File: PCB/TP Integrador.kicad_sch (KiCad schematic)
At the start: 33 parts, among them Q1 BC547C, Q10 BC547C, Q11 BC547C, Q2 2N3019, Q3 D45H11, Q4 BC547C, Q5 BC557C, Q6 BC557C, Q7 BC547C, Q8 BC557C, Q9 BC547C

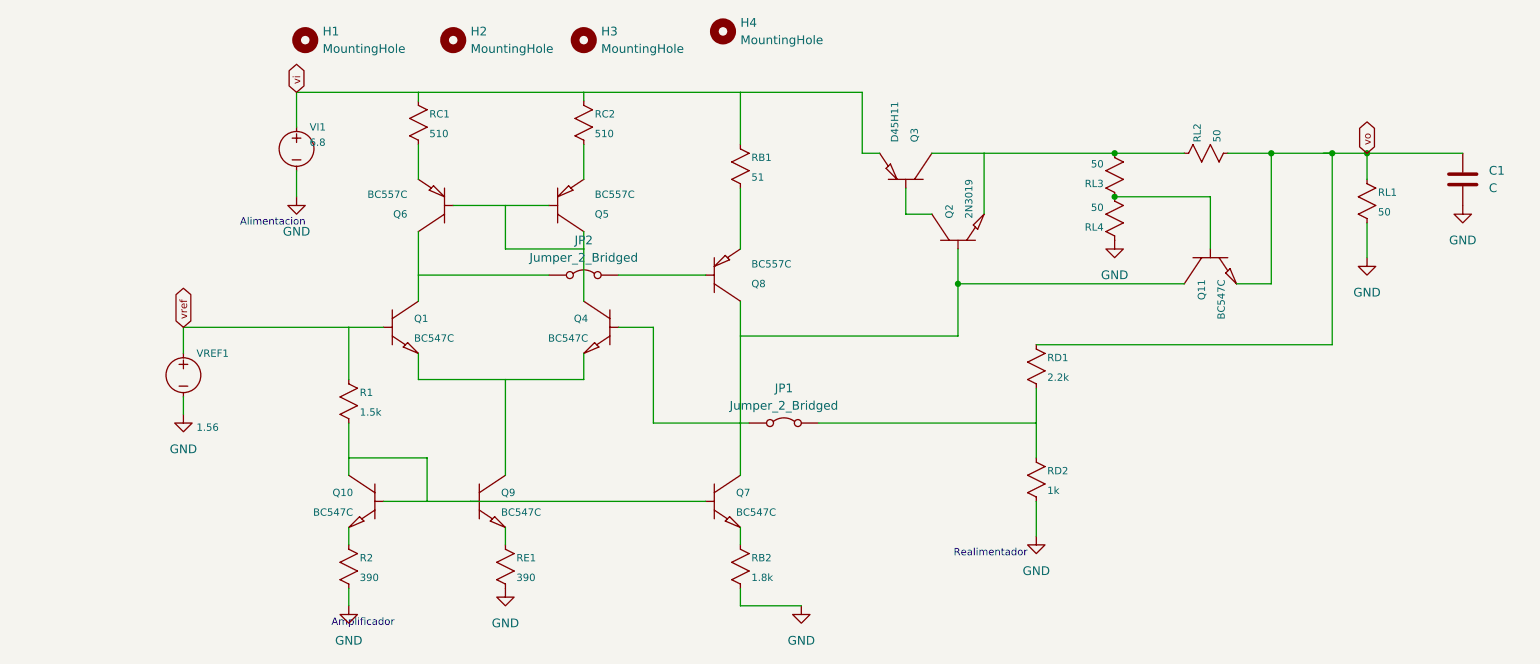
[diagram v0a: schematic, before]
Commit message: Update checkpoint 2
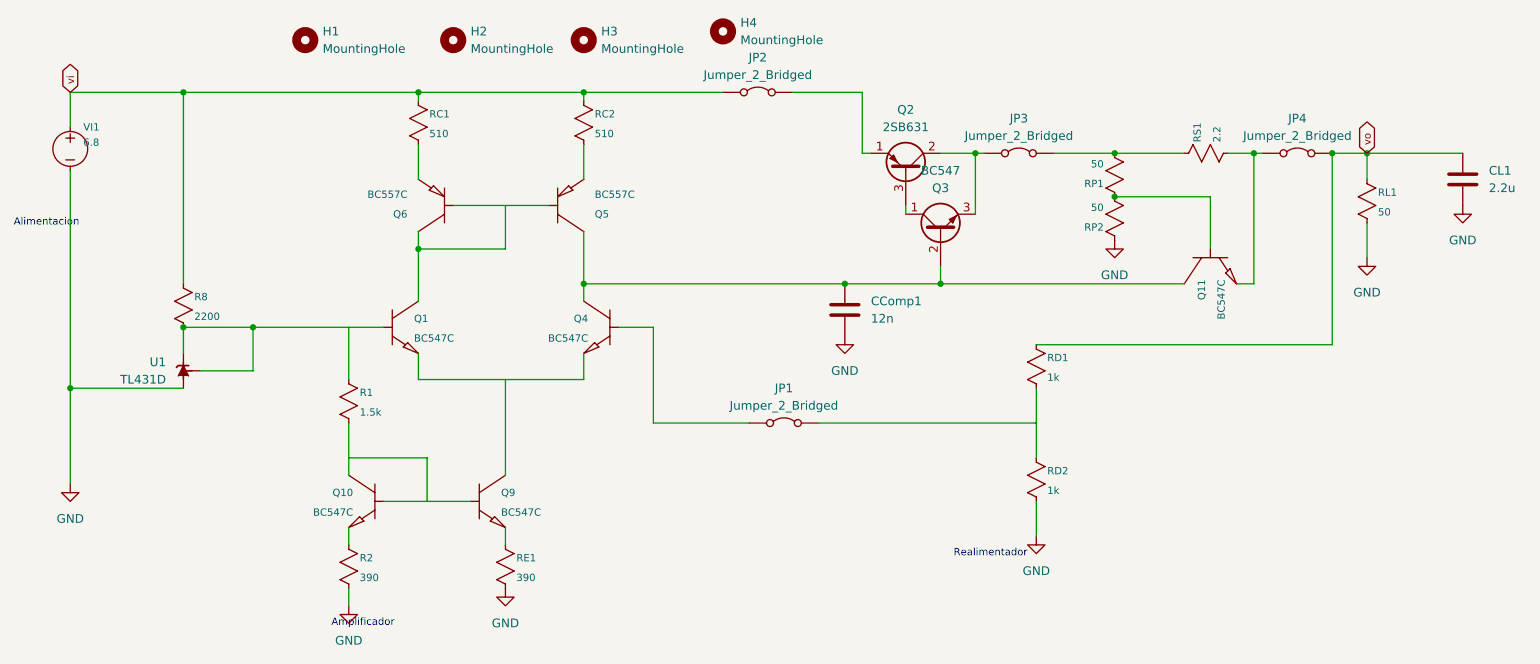
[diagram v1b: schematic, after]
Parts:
- removed Q2: 2N3019, Package_TO_SOT_THT:TO-39-3, symbol ltspice:npn
- removed Q3: D45H11, Package_TO_SOT_THT:TO-220-3_Vertical, symbol ltspice:pnp
- removed Q7: BC547C, Package_TO_SOT_THT:TO-92_Inline_Wide, symbol ltspice:npn
- removed Q8: BC557C, Package_TO_SOT_THT:TO-92_Inline_Wide, symbol ltspice:pnp
- removed RB1: 51, Resistor_THT:R_Axial_DIN0207_L6.3mm_D2.5mm_P7.62mm_Horizontal, symbol ltspice:res
- removed RB2: 1.8k, Resistor_THT:R_Axial_DIN0207_L6.3mm_D2.5mm_P7.62mm_Horizontal, symbol ltspice:res
- removed VREF1: 1.56, TerminalBlock_Phoenix:TerminalBlock_Phoenix_MKDS-1,5-2-5.08_1x02_P5.08mm_Horizontal, symbol ltspice:voltage
- added CComp1: 12n, Capacitor_THT:CP_Radial_D4.0mm_P1.50mm, symbol Device:C
- added JP3, JP4: Jumper_2_Bridged, TestPoint:TestPoint_2Pads_Pitch5.08mm_Drill1.3mm, symbol Jumper:Jumper_2_Bridged
- added Q2: 2SB631, Package_TO_SOT_THT:TO-126-3_Vertical, symbol Transistor_BJT:2SB631
- added Q3: BC547, Package_TO_SOT_THT:TO-92_Inline_Wide, symbol Transistor_BJT:BC547
- added R8: 2200, Resistor_THT:R_Axial_DIN0207_L6.3mm_D2.5mm_P7.62mm_Horizontal, symbol ltspice:res
- added U1: TL431D, Package_TO_SOT_THT:TO-92_Inline_Wide, symbol Reference_Voltage:TL431D
- CL1: renamed from C1; value C -> 2.2u
- RD1: value 2.2k -> 1k
- RS1: renamed from RL2; value 50 -> 2.2
- renumbered RL3 to RP1, RL4 to RP2
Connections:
- net GND: now also CComp1.2, U1.2 (A), U1.3 (A), U1.6 (A), U1.7 (A)
- net vi: now also JP2.1 (A), R8.1
- net vo: now also JP4.2 (B); no longer Q11.3 (E), RS1.2
- net at Q11.1 (C): now also Q4.1 (C), Q5.1 (C), CComp1.1, Q3.2 (B)
- net at RP1.2, RS1.1: now also JP3.2 (B)
- net at Q5.2 (B), Q6.2 (B): now also Q1.1 (C), Q6.1 (C); no longer Q4.1 (C), Q5.1 (C)
- net at JP2.2 (B): now also Q2.1 (E)
- net vref: no longer names the net of Q1.2 (B), R1.1
- net vref: now also R8.2, U1.1 (K), U1.8 (REF)
- new net: JP3.1 (A), Q2.2 (C), Q3.3 (E)
- new net: Q2.3 (B), Q3.1 (C)
- new net: JP4.1 (A), Q11.3 (E), RS1.2
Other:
- moved on the sheet: JP2, VI1
